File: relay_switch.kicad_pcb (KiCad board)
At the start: 2 copper layers, 25.6 x 60.4 mm, 18 parts, among them P1 board_mount, P10 INPUT2, P11 INPUT3, P12 INPUT4, P13 12vdc, P14 J_CONN_01X04, P2 board_mount, P3 board_mount, P4 board_mount, P8 OUTPUT, P9 INPUT1, U1 ULN2003A

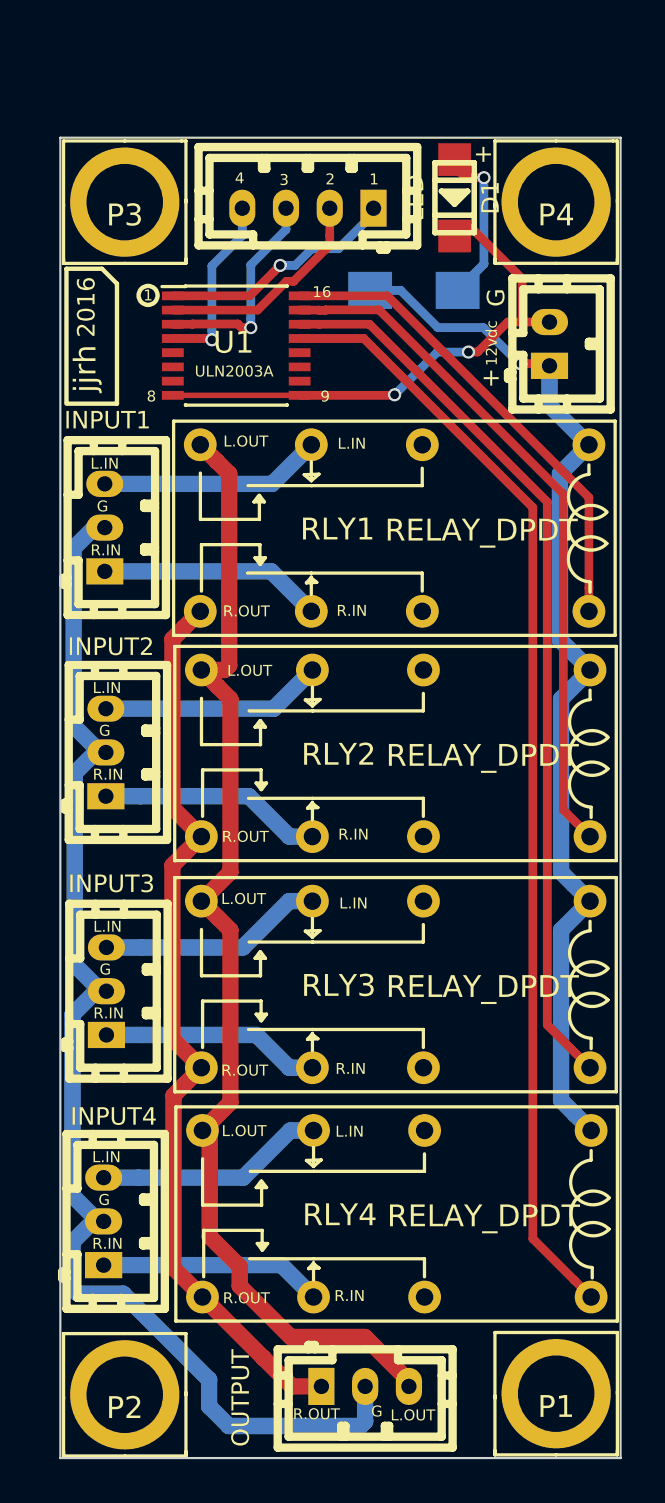
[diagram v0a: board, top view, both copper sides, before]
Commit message: board changes and corrections
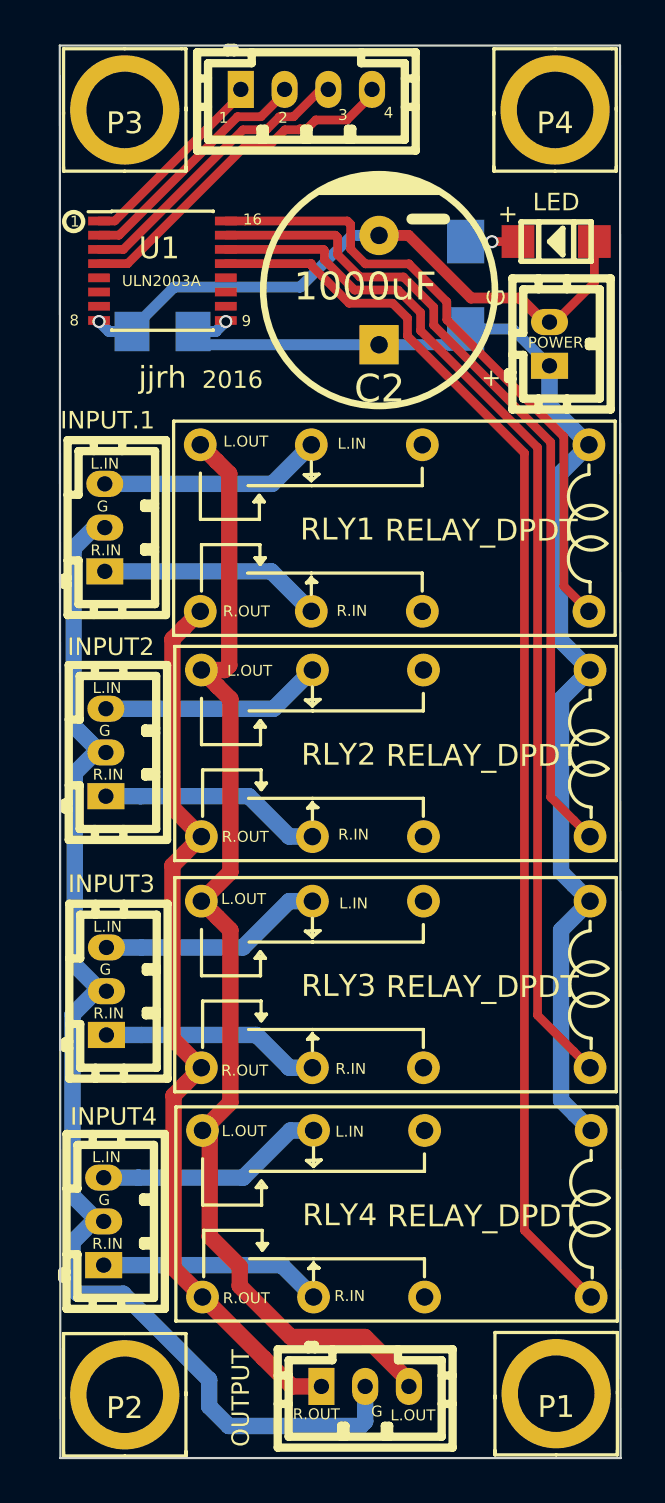
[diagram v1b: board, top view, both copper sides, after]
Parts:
- added C1: 100nF, w_smd_cap:c_1206, B.Cu at (136.2, 117.3)
- added C2: 1000uF, w_capacitors:CP_10x20mm, F.Cu at (146.1, 115.4)
- P13: value 12vdc -> POWER
- P9: value INPUT1 -> INPUT.1
- moved P14 5.44 mm to (142.8, 106.2), turned to 0 degrees
- moved D1 5.06 mm to (154.2, 113.2), turned to 180 degrees
- moved U1 4.81 mm to (136.2, 114.5)
- moved P3 4.22 mm to (134.5, 107.3)
- moved P4 4.22 mm to (154.2, 107.3)
- moved R1 2.38 mm to (150.1, 115.2), turned to 90 degrees
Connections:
- net G_OUT renamed R1_GND
- D1 pad 1: Net-(D1-Pad1) -> GND
- D1 pad 2: GND -> Net-(D1-Pad2)
- R1 pad 2: Net-(D1-Pad1) -> Net-(D1-Pad2)
- U1 pad 9: GND -> +12V
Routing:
- net +12V: track 48.7 -> 58.4 mm
- net Net-(D1-Pad1): track 7.34 -> 0.00 mm, vias 1 -> 0
- net T4: track 8.78 -> 15.9 mm, vias 1 -> 0
- net Net-(RLY1-Pad1): track 22.3 -> 29.2 mm
- net Net-(RLY2-Pad1): track 31.7 -> 38.5 mm
- net Net-(RLY3-Pad1): track 41.4 -> 48.1 mm
- net Net-(RLY4-Pad1): track 51.1 -> 57.7 mm
- net GND: track 24.6 -> 29.1 mm, vias 2 -> 1
- net T3: track 10.0 -> 13.5 mm, vias 1 -> 0
- net Net-(D1-Pad2): track 0.00 -> 2.40 mm, vias 0 -> 1
- net T1: track 11.0 -> 9.13 mm, vias 1 -> 0
- net T2: track 10.1 -> 11.3 mm
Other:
- board size 25.6 x 60.4 mm -> 25.7 x 64.6 mm
